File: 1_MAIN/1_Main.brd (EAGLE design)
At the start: 67.4 x 54.8 mm, 40 parts, among them IC1 NCP1117-33ST, IC10 FT232RL, IC7 MAX14932, IC8 MAX14932, IC9 MAX14932, Q1 IRF7416, X14 ALLSERIALMM, X2 MINI-USB-32005-201, X3 AKL18X-04W

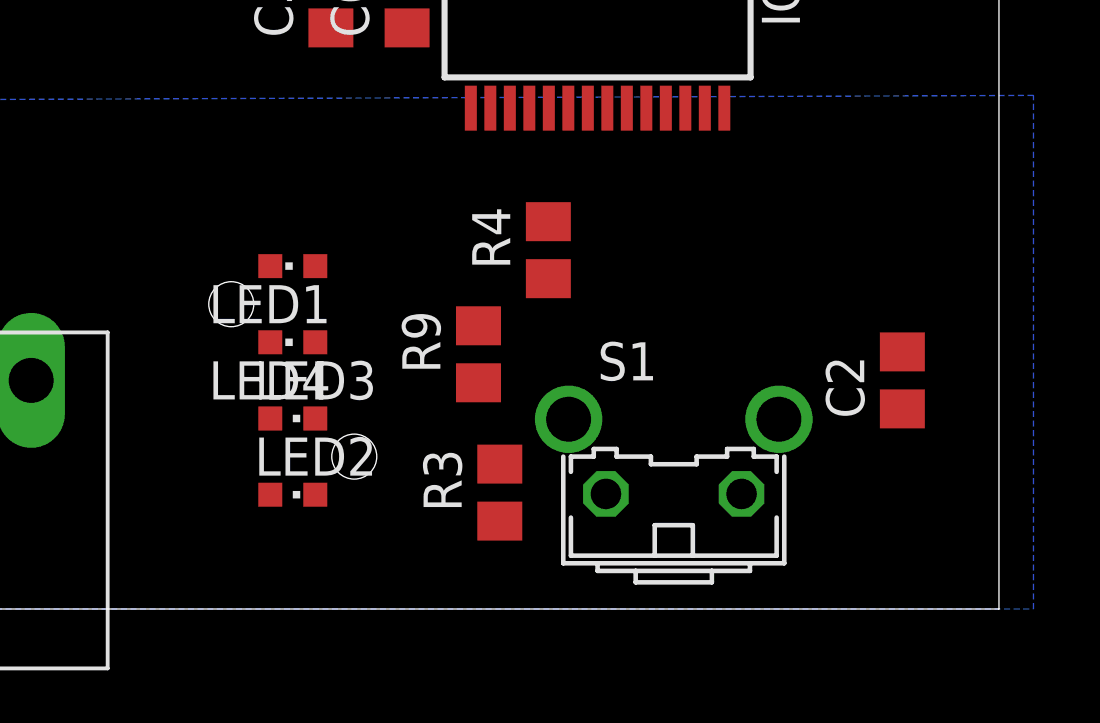
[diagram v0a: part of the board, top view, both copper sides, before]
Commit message: updated readme & mainboard
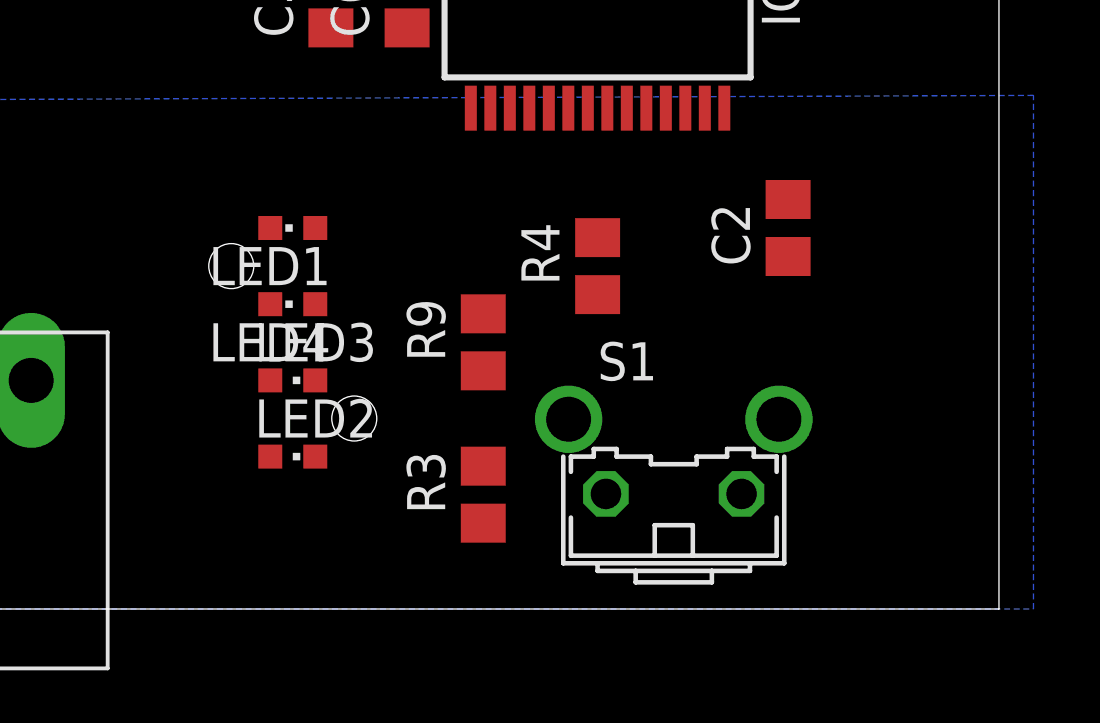
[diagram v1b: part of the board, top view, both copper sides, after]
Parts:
- moved C2 6.35 mm to (26.7, 12.7)
- moved R4 1.72 mm to (20.3, 11.4)
- moved LED3 1.27 mm to (10.2, 7.62)
- moved U$3 1.27 mm to (10.2, 8.89)
- moved LED2 1.27 mm to (10.2, 5.08)
- moved LED1 1.27 mm to (10.2, 12.7)
- moved LED4 1.27 mm to (10.2, 10.2)
- moved R3 0.55 mm to (16.5, 3.81)
- moved R9 0.43 mm to (16.5, 8.89)
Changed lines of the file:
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@@
 <elements>
 <element name="L10" library="EagleLibrary_Wuerth_Elektronik_eiSos_Version_6-12" package="0805" value="WE-CBF_0805" x="-23.38" y="12.74" rot="R90"/>
-<element name="R3" library="rcl" package="R0805" value="270" x="17.06" y="3.88" rot="R90"/>
-<element name="R4" library="rcl" package="R0805" value="270" x="18.68" y="11.96" rot="R90"/>
-<element name="LED2" library="led" package="CHIPLED_0603" value="RX" x="10.16" y="3.81" rot="R270">
-<attribute name="COLOR" value="GN" x="10.16" y="3.81" size="1.778" layer="27" rot="R270" display="off"/>
-</element>
-<element name="LED3" library="led" package="CHIPLED_0603" value="TX" x="10.16" y="6.35" rot="R270">
-<attribute name="COLOR" value="RD" x="10.16" y="6.35" size="1.778" layer="27" rot="R270" display="off"/>
+<element name="R3" library="rcl" package="R0805" value="270" x="16.51" y="3.81" rot="R90"/>
+<element name="R4" library="rcl" package="R0805" value="270" x="20.32" y="11.43" rot="R90"/>
+<element name="LED2" library="led" package="CHIPLED_0603" value="RX" x="10.16" y="5.08" rot="R270">
+<attribute name="COLOR" value="GN" x="10.16" y="5.08" size="1.778" layer="27" rot="R270" display="off"/>
+</element>
+<element name="LED3" library="led" package="CHIPLED_0603" value="TX" x="10.16" y="7.62" rot="R270">
+<attribute name="COLOR" value="RD" x="10.16" y="7.62" size="1.778" layer="27" rot="R270" display="off"/>
 </element>
 <element name="C1" library="rcl" package="C0805" value="10n" x="-26.67" y="11.43" rot="R180"/>
-<element name="C2" library="rcl" package="C0805" value="100n" x="30.48" y="7.62" rot="R90"/>
+<element name="C2" library="rcl" package="C0805" value="100n" x="26.67" y="12.7" rot="R90"/>
 <element name="C3" library="rcl" package="C0805" value="10µ" x="30.48" y="40.64" rot="R90"/>
 <element name="R8" library="rcl" package="R0805" value="180" x="30.48" y="25.4"/>
-<element name="LED1" library="led" package="CHIPLED_0603" value="PWR" x="10.16" y="11.43" rot="R90">
-<attribute name="COLOR" value="GN" x="10.16" y="11.43" size="1.778" layer="27" rot="R90" display="off"/>
+<element name="LED1" library="led" package="CHIPLED_0603" value="PWR" x="10.16" y="12.7" rot="R90">
+<attribute name="COLOR" value="GN" x="10.16" y="12.7" size="1.778" layer="27" rot="R90" display="off"/>
 </element>
 <element name="C13" library="rcl" package="C0805" value="10µ" x="30.85" y="35.56" rot="R90"/>
@@
 </element>
 <element name="C18" library="rcl" package="C0805" value="100n" x="31.75" y="30.48" rot="R270"/>
-<element name="R9" library="rcl" package="R0805" value="180" x="16.35" y="8.49" rot="R90"/>
-<element name="LED4" library="led" package="CHIPLED_0603" value="TXEN" x="10.16" y="8.89" rot="R90">
-<attribute name="COLOR" value="YE" x="10.16" y="8.89" size="1.778" layer="27" rot="R90" display="off"/>
+<element name="R9" library="rcl" package="R0805" value="180" x="16.51" y="8.89" rot="R90"/>
+<element name="LED4" library="led" package="CHIPLED_0603" value="TXEN" x="10.16" y="10.16" rot="R90">
+<attribute name="COLOR" value="YE" x="10.16" y="10.16" size="1.778" layer="27" rot="R90" display="off"/>
 </element>
 <element name="X2" library="con-cypressindustries" package="32005-201" value="MINI-USB-32005-201" x="-21.59" y="5.08" rot="R90">
@@
 <attribute name="OC_FARNELL" value="unknown" x="3.81" y="26.67" size="1.778" layer="27" display="off"/>
 </element>
-<element name="U$3" library="Mentor" package="1296.1004" value="" x="10.16" y="7.62" rot="R180"/>
+<element name="U$3" library="Mentor" package="1296.1004" value="" x="10.16" y="8.89" rot="R180"/>
 <element name="IC7" library="max14932" package="SO16" value="MAX14932" x="-8.89" y="35.56"/>
 <element name="IC8" library="max14932" package="SO16" value="MAX14932" x="7.62" y="35.56"/>
@@
 <wire x1="22.595" y1="16.695" x2="19.995" y2="16.695" width="0" layer="19" extent="1-1"/>
 <wire x1="20.645" y1="23.945" x2="13.97" y2="21.27" width="0" layer="19" extent="1-1"/>
-<wire x1="9.41" y1="11.43" x2="11.43" y2="21.27" width="0" layer="19" extent="1-1"/>
-<wire x1="9.41" y1="8.89" x2="9.41" y2="11.43" width="0" layer="19" extent="1-1"/>
-<wire x1="20.5994" y1="3.8354" x2="9.41" y2="8.89" width="0" layer="19" extent="1-1"/>
+<wire x1="9.41" y1="12.7" x2="11.43" y2="21.27" width="0" layer="19" extent="1-1"/>
+<wire x1="9.41" y1="10.16" x2="9.41" y2="12.7" width="0" layer="19" extent="1-1"/>
 <wire x1="31.75" y1="29.53" x2="20.645" y2="23.945" width="0" layer="19" extent="1-1"/>
+<wire x1="20.5994" y1="3.8354" x2="19.995" y2="16.695" width="0" layer="19" extent="1-1"/>
 <wire x1="-19.99" y1="8.08" x2="-12.065" y2="32.96" width="0" layer="19" extent="1-1"/>
 <wire x1="-27.62" y1="11.43" x2="-19.99" y2="8.08" width="0" layer="19" extent="1-1"/>
@@
 <contactref element="IC10" pad="23"/>
 <contactref element="R4" pad="2"/>
-<wire x1="18.68" y1="12.91" x2="21.295" y2="16.695" width="0" layer="19" extent="1-1"/>
+<wire x1="20.32" y1="12.38" x2="21.295" y2="16.695" width="0" layer="19" extent="1-1"/>
 </signal>
 <signal name="RXLED">
 <contactref element="IC10" pad="22"/>
 <contactref element="R3" pad="2"/>
-<wire x1="17.06" y1="4.83" x2="20.645" y2="16.695" width="0" layer="19" extent="1-1"/>
+<wire x1="16.51" y1="4.76" x2="20.645" y2="16.695" width="0" layer="19" extent="1-1"/>
 </signal>
 <signal name="N$38">
@@
 <wire x1="-22.86" y1="20" x2="-24.765" y2="21.65" width="0" layer="19" extent="1-1"/>
 <wire x1="31.43" y1="25.4" x2="22.54" y2="39.37" width="0" layer="19" extent="1-1"/>
-<wire x1="9.41" y1="6.35" x2="10.795" y2="32.96" width="0" layer="19" extent="1-1"/>
-<wire x1="9.41" y1="3.81" x2="9.41" y2="6.35" width="0" layer="19" extent="1-1"/>
+<wire x1="9.41" y1="7.62" x2="10.795" y2="32.96" width="0" layer="19" extent="1-1"/>
+<wire x1="9.41" y1="5.08" x2="9.41" y2="7.62" width="0" layer="19" extent="1-1"/>
 </signal>
 <signal name="N$5">
@@
 <contactref element="R4" pad="1"/>
 <contactref element="LED3" pad="C"/>
-<wire x1="10.91" y1="6.35" x2="18.68" y2="11.01" width="0" layer="19" extent="1-1"/>
+<wire x1="10.91" y1="7.62" x2="20.32" y2="10.48" width="0" layer="19" extent="1-1"/>
 </signal>
 <signal name="N$6">
 <contactref element="R3" pad="1"/>
 <contactref element="LED2" pad="C"/>
-<wire x1="10.91" y1="3.81" x2="17.06" y2="2.93" width="0" layer="19" extent="1-1"/>
+<wire x1="10.91" y1="5.08" x2="16.51" y2="2.86" width="0" layer="19" extent="1-1"/>
 </signal>
 <signal name="N$7">
 <contactref element="R9" pad="1"/>
 <contactref element="LED4" pad="A"/>
-<wire x1="10.91" y1="8.89" x2="16.35" y2="7.54" width="0" layer="19" extent="1-1"/>
+<wire x1="10.91" y1="10.16" x2="16.51" y2="7.94" width="0" layer="19" extent="1-1"/>
 </signal>
 <signal name="N$8">
 <contactref element="R8" pad="1"/>
 <contactref element="LED1" pad="A"/>
-<wire x1="10.91" y1="11.43" x2="29.53" y2="25.4" width="0" layer="19" extent="1-1"/>
+<wire x1="10.91" y1="12.7" x2="29.53" y2="25.4" width="0" layer="19" extent="1-1"/>
 </signal>
 <signal name="GND1">
@@
 <wire x1="-11.43" y1="42.545" x2="-12.065" y2="38.16" width="0" layer="19" extent="1-1"/>
 <wire x1="-27.7114" y1="29.9212" x2="-19.05" y2="40.64" width="0" layer="19" extent="1-1"/>
-<wire x1="30.48" y1="8.57" x2="30.85" y2="36.51" width="0" layer="19" extent="1-1"/>
+<wire x1="26.67" y1="13.65" x2="30.85" y2="36.51" width="0" layer="19" extent="1-1"/>
 <wire x1="-9.06" y1="7.62" x2="-2.54" y2="35.88" width="0" layer="19" extent="1-1"/>
 </signal>
@@
 <wire x1="-8.89" y1="46.99" x2="-8.89" y2="45.085" width="0.4064" layer="1"/>
 <contactref element="IC1" pad="3"/>
-<wire x1="30.48" y1="6.67" x2="30.48" y2="39.69" width="0" layer="19" extent="1-1"/>
-<wire x1="-2.06" y1="7.62" x2="30.48" y2="6.67" width="0" layer="19" extent="1-1"/>
+<wire x1="26.67" y1="11.75" x2="30.48" y2="39.69" width="0" layer="19" extent="1-1"/>
+<wire x1="-2.06" y1="7.62" x2="26.67" y2="11.75" width="0" layer="19" extent="1-1"/>
 <wire x1="-23.0886" y1="29.9212" x2="-2.06" y2="7.62" width="0" layer="19" extent="1-1"/>
 <wire x1="-16.51" y1="48.26" x2="-23.0886" y2="29.9212" width="0" layer="19" extent="1-1"/>
@@
 <contactref element="IC9" pad="3"/>
 <wire x1="16.745" y1="23.945" x2="22.92" y2="43.815" width="0" layer="19" extent="1-1"/>
-<wire x1="16.35" y1="9.44" x2="16.745" y2="23.945" width="0" layer="19" extent="1-1"/>
+<wire x1="16.51" y1="9.84" x2="16.745" y2="23.945" width="0" layer="19" extent="1-1"/>
 </signal>
 <signal name="N$13">

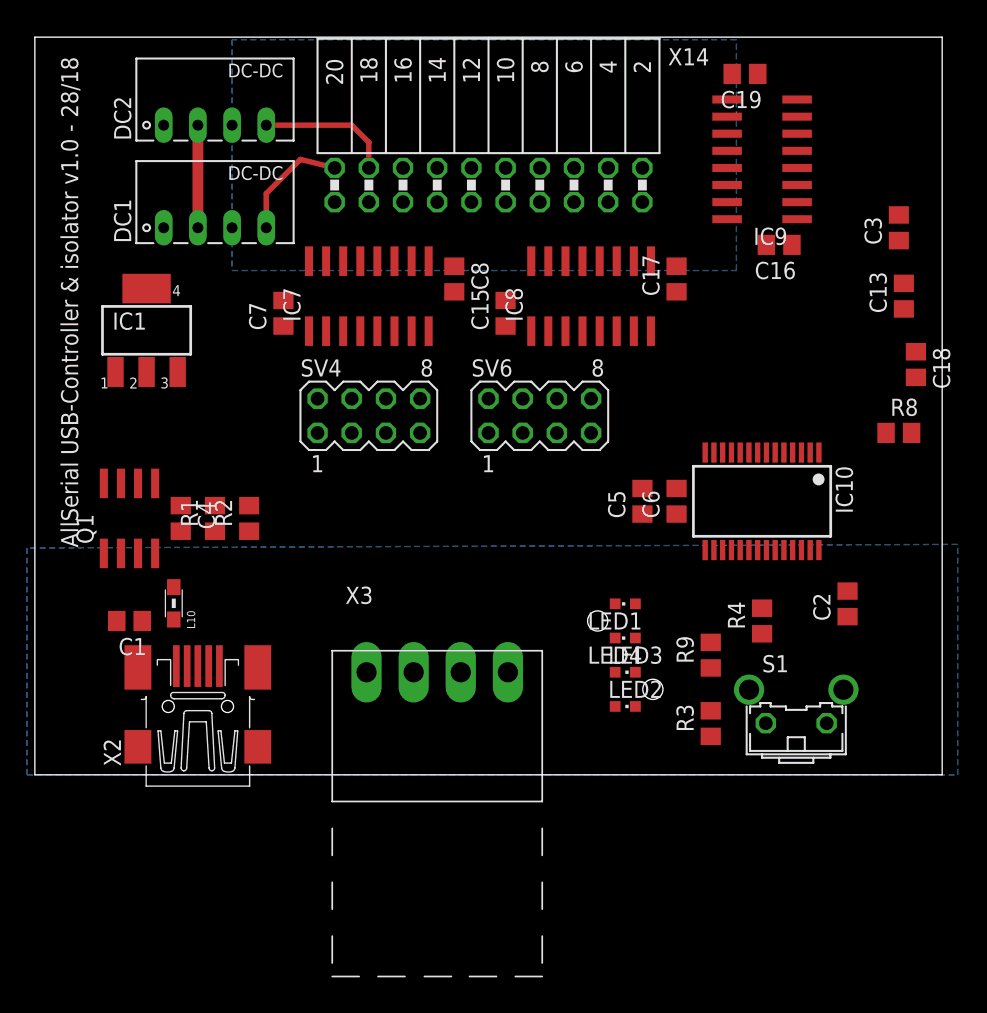
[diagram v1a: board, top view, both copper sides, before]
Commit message: finish FTDI PCB
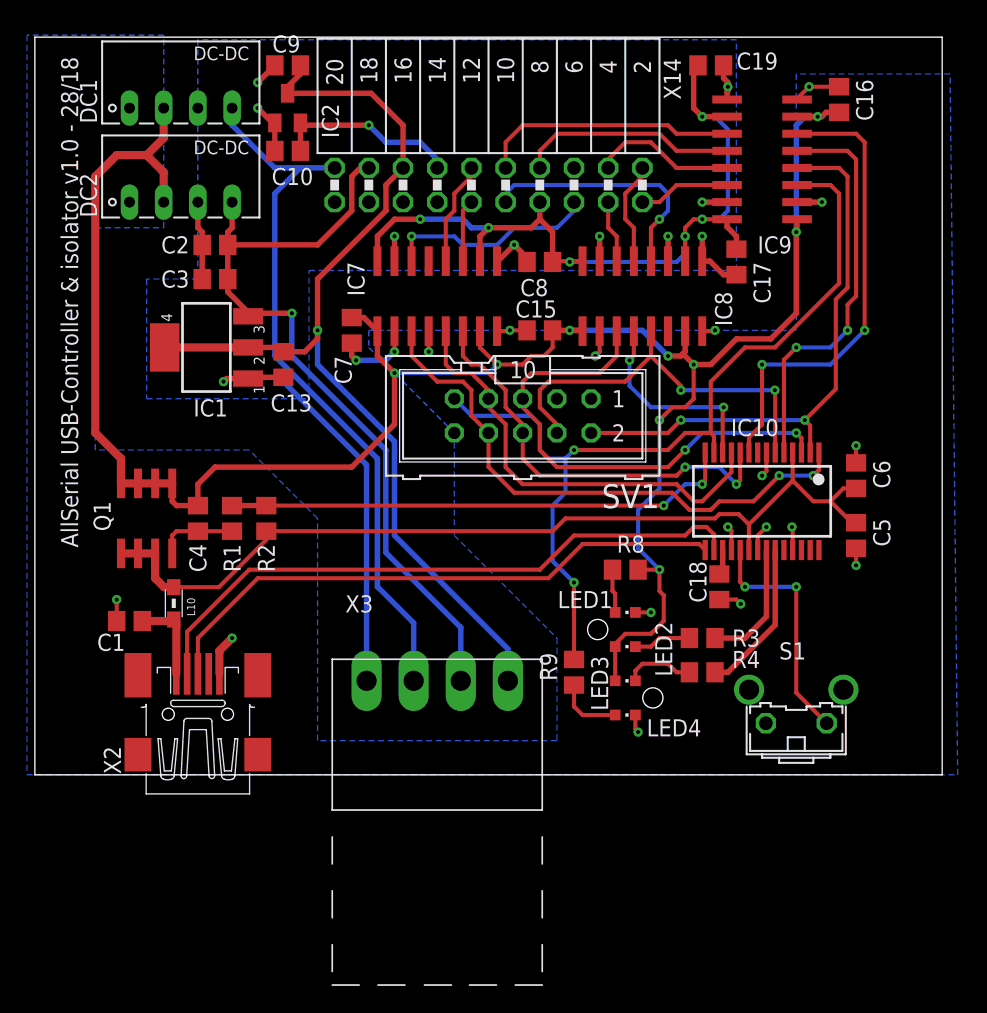
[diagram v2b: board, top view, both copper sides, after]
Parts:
- removed SV4, SV6: (no value), con-lstb:MA04-2
- added C10, C9: 1µ, rcl:C0805
- added IC2: MCP1700T-1802E, SeeSys:SOT23
- added SV1: (no value), con-harting-ml:ML10
- moved C2 54.0 mm to (-20.3, 39.4), turned to 180 degrees
- moved C3 50.9 mm to (-20.3, 36.8), turned to 180 degrees
- moved C13 46.4 mm to (-15.2, 30.5), turned to 270 degrees
- moved R8 22.7 mm to (10.2, 15.2)
- moved C18 22.0 mm to (17.1, 14.0)
- moved C5 16.1 mm to (27.3, 17.8), turned to 270 degrees
- moved C6 13.5 mm to (27.3, 22.2)
- moved C16 11.7 mm to (26.0, 50.2), turned to 90 degrees
- moved R9 10.2 mm to (6.35, 7.62)
- moved DC1 9.25 mm to (-22.9, 49.5)
- moved C8 6.48 mm to (3.81, 38.1), turned to 180 degrees
- moved R3 6.38 mm to (15.9, 10.2), turned to 0 degrees
- moved DC2 6.25 mm to (-22.9, 42.5)
- moved R4 5.85 mm to (15.9, 7.62), turned to 0 degrees
- moved LED4 5.71 mm to (10.2, 4.45), turned to 270 degrees
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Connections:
- new net +1V8/1: C10.1, IC2.2, X14.14
- net +3V3/1: now also C9.1, IC2.3
- net GND: now also IC7.4, SV1.10; no longer IC9.4
- net GND1: now also C10.2, C9.2, IC2.1, IC8.11; no longer IC9.11
- net N$14: now also SV1.8
- net N$29: now also SV1.5
- net N$3: now also SV1.9
- net N$32: now also SV1.7
- net N$33: now also IC9.4, SV1.2; no longer IC7.4
- net N$34: now also IC9.6; no longer IC8.5
- net N$35: now also SV1.6
- net N$36: now also IC8.5, SV1.4; no longer IC8.6
- net N$84: now also IC9.13; no longer IC7.13
- net N$85: now also IC9.11; no longer IC8.12
- net N$87: now also IC8.12; no longer IC8.11
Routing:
- net +5V: track 7.62 -> 162.4 mm, vias 0 -> 9
- net +3V3/1: track 0.00 -> 74.3 mm, vias 0 -> 1
- net N$38: track 0.00 -> 68.6 mm
- net N$3: track 0.00 -> 66.7 mm, vias 0 -> 2
- net VIN1: track 0.00 -> 59.9 mm, vias 0 -> 6
- net GND1: track 0.00 -> 59.1 mm, vias 0 -> 10
- net +5V/1: track 10.1 -> 59.4 mm, vias 0 -> 1
- net N$19: track 0.00 -> 46.9 mm
- net +12V/1: track 8.75 -> 53.4 mm
- net N$21: track 0.00 -> 43.4 mm
- net N$33: track 0.00 -> 42.3 mm, vias 0 -> 2
- net N$14: track 0.00 -> 42.0 mm, vias 0 -> 2
- net !PWEN: track 0.00 -> 38.0 mm, vias 0 -> 2
- net N$29: track 0.00 -> 37.5 mm, vias 0 -> 2
- net GND: track 0.00 -> 37.0 mm, vias 0 -> 19
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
